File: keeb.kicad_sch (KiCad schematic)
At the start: 20 parts, among them SW1 SW_Push, U1 ATmega32U4-A, Y1 16MHz

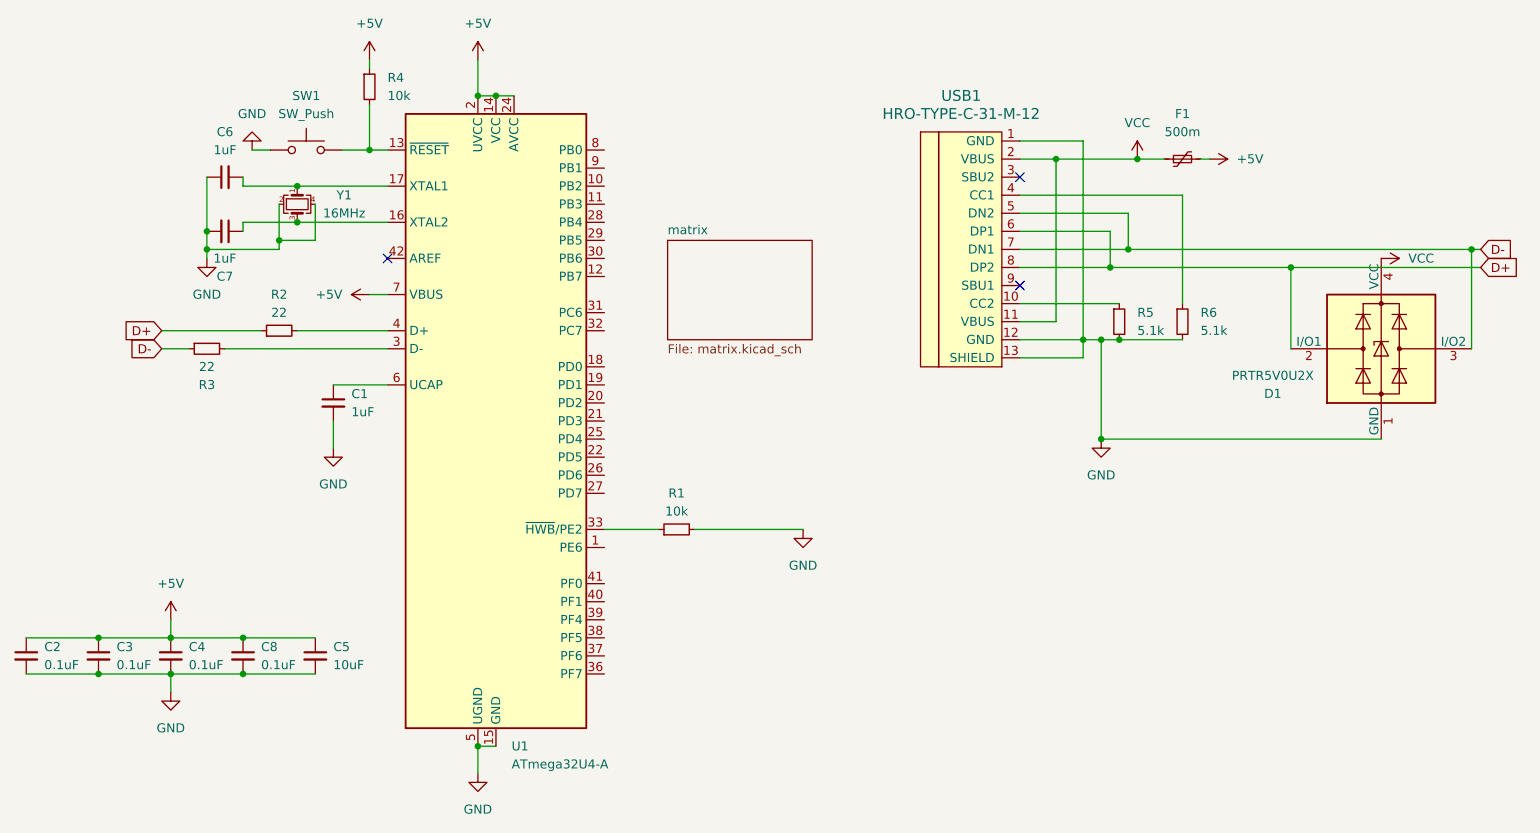
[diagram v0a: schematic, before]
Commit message: arcade session 3
added footprints; lots of errors :( problem for next time i am free
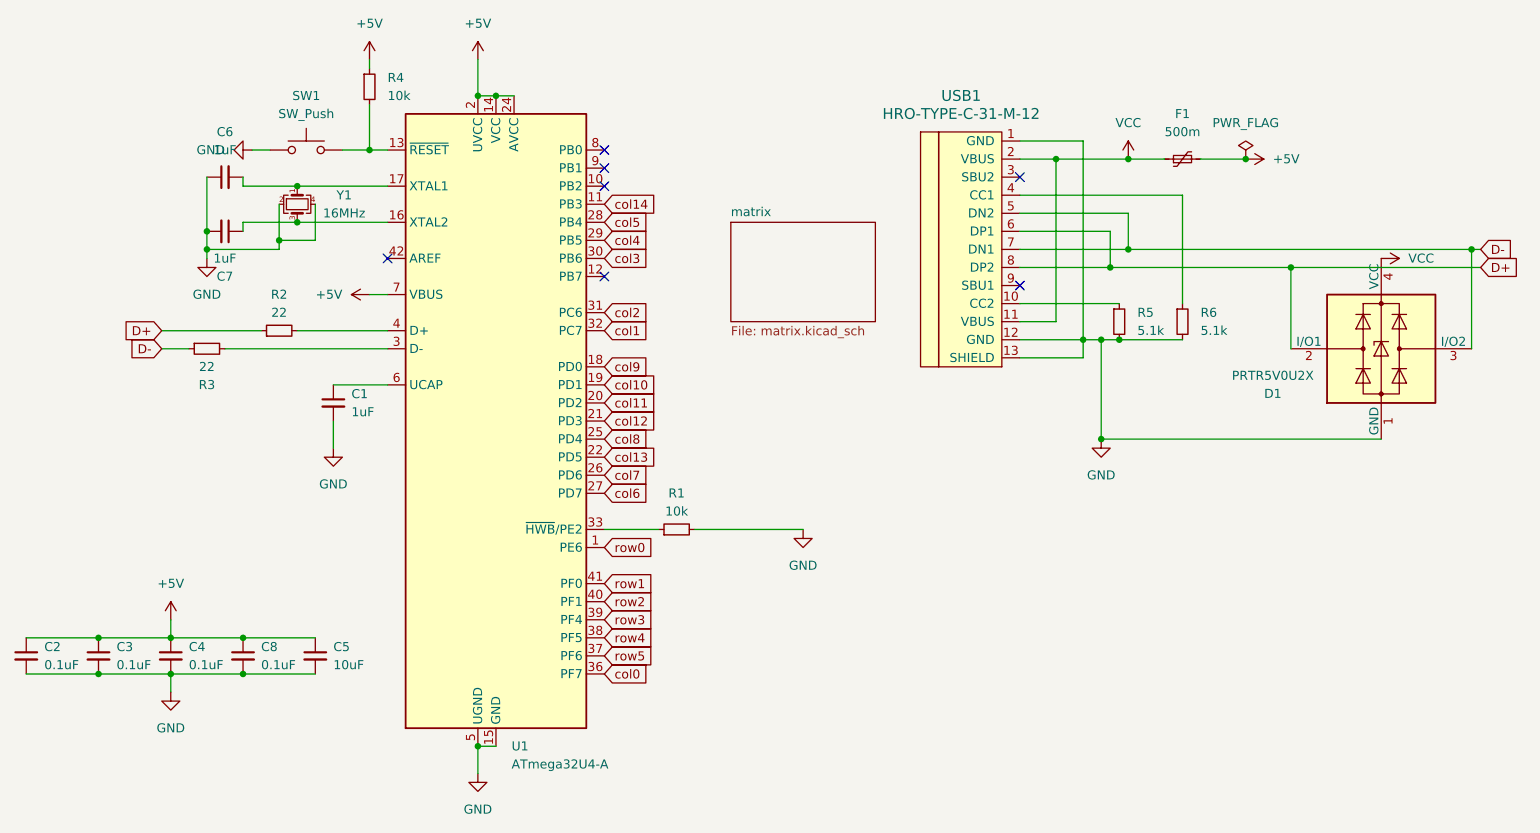
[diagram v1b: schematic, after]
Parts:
- C1, C2, C3, C4, C5, C6, C7, C8: footprint (none) -> Capacitor_SMD:C_0805_2012Metric
- F1: footprint (none) -> Fuse:Fuse_1206_3216Metric_Pad1.42x1.75mm_HandSolder
- R1, R2, R3, R4, R5, R6: footprint (none) -> Resistor_SMD:R_0805_2012Metric
- SW1: footprint (none) -> Button_Switch_SMD:SW_SPST_SKQG_WithStem
- USB1: footprint (none) -> Type-C:Wurth-632723300011-HandSoldering
- Y1: footprint (none) -> Crystal:Crystal_SMD_3225-4Pin_3.2x2.5mm_HandSoldering
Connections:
- net row0: now reaches U1.1 (PE6)
- net col14: now reaches U1.11 (PB3)
- net col9: now reaches U1.18 (PD0)
- net col10: now reaches U1.19 (PD1)
- net col11: now reaches U1.20 (PD2)
- net col12: now reaches U1.21 (PD3)
- net col13: now reaches U1.22 (PD5)
- net col8: now reaches U1.25 (PD4)
- net col7: now reaches U1.26 (PD6)
- net col6: now reaches U1.27 (PD7)
- net col5: now reaches U1.28 (PB4)
- net col4: now reaches U1.29 (PB5)
- net col3: now reaches U1.30 (PB6)
- net col2: now reaches U1.31 (PC6)
- net col1: now reaches U1.32 (PC7)
- net col0: now reaches U1.36 (PF7)
- net row5: now reaches U1.37 (PF6)
- net row4: now reaches U1.38 (PF5)
- net row3: now reaches U1.39 (PF4)
- net row2: now reaches U1.40 (PF1)
- net row1: now reaches U1.41 (PF0)
- no-connect marks 3 -> 7
